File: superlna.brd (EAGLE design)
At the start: 41.2 x 21.8 mm, 14 parts, among them U1 BIASTEE, X1 SMA-142-0701-801/806, X2 SMA-142-0701-801/806

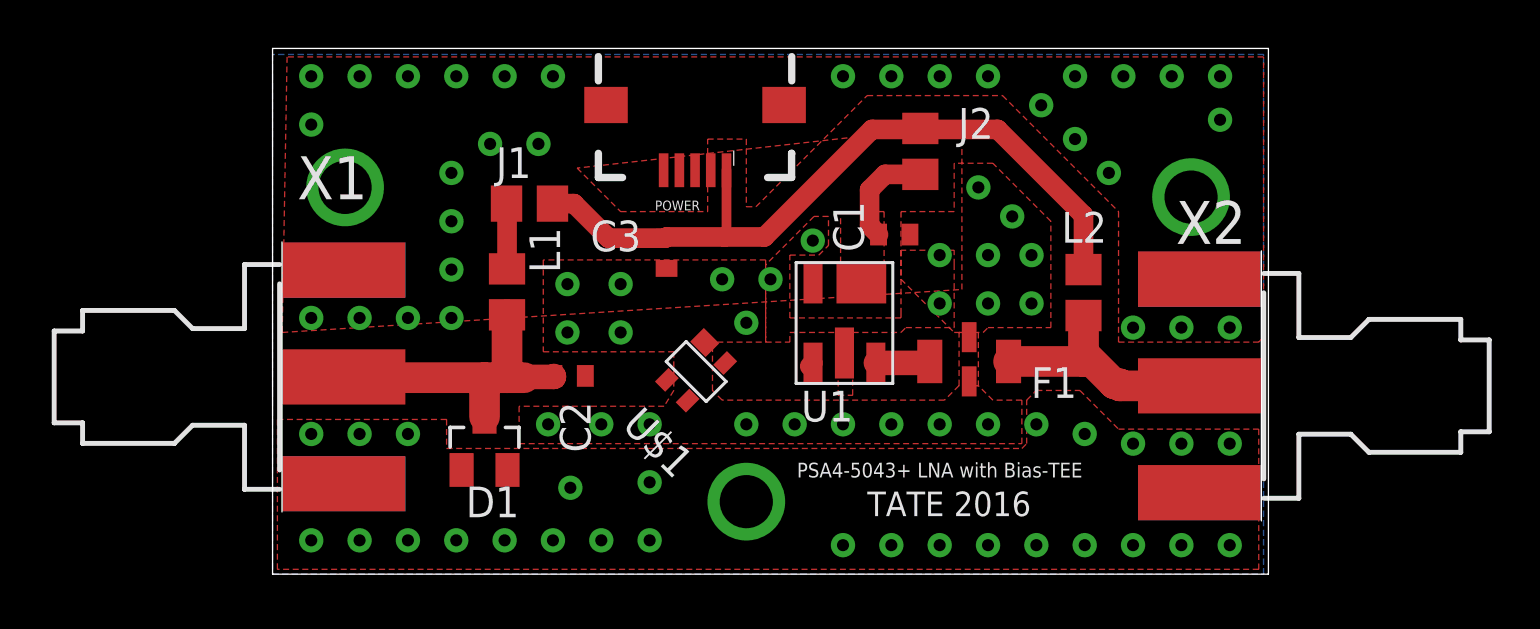
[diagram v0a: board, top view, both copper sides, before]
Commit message: V2
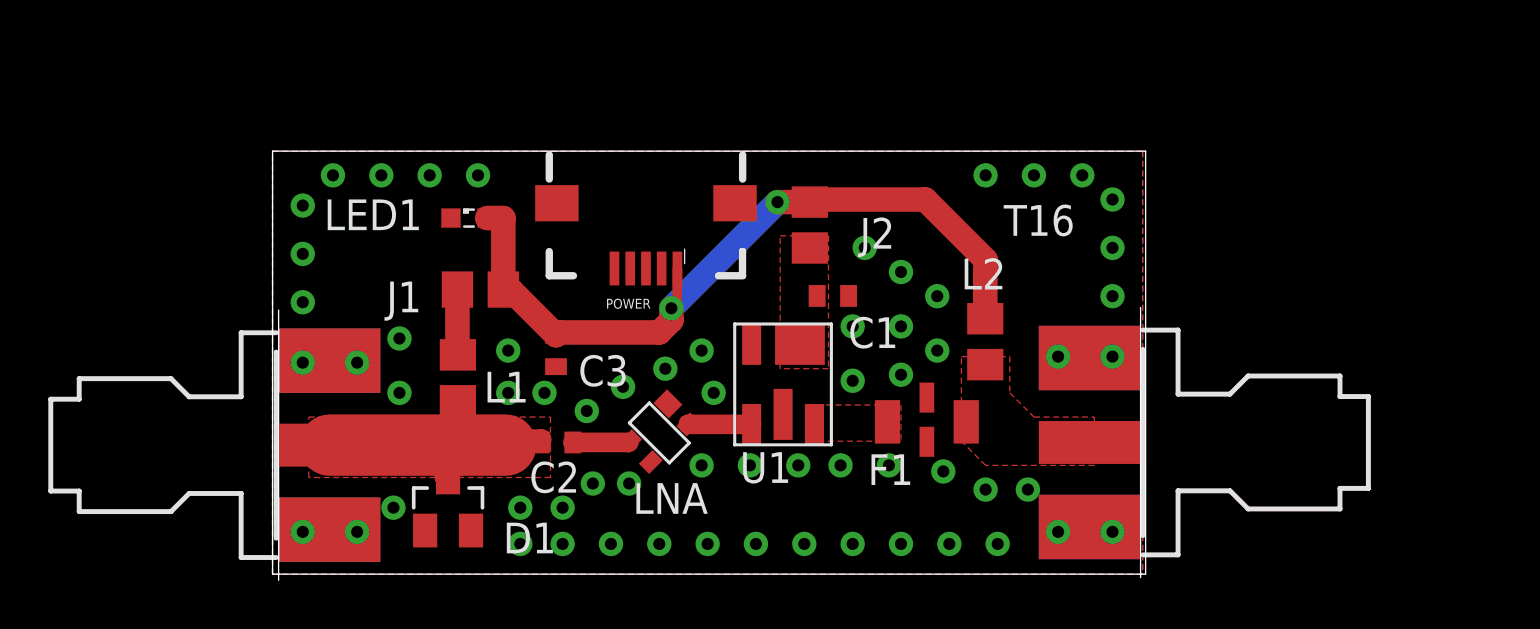
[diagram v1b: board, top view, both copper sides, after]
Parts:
- removed U$1: AMP, minicircuits:SOC-343
- removed X2: SMA-142-0701-801/806, con-coax:J502-ND-142-0701-801/806
- added LED1: (no value), eagle-ltspice:LED_SML0603
- added LNA: AMP, minicircuits:SOC-343
- added RFIN: SMA-142-0711-821/826, con-coax:J502-ND-142-0711-821/826
- X1: value SMA-142-0701-801/806 -> SMA-142-0711-821/826; device con-coax:J502-ND-142-0701-801/806 -> con-coax:J502-ND-142-0711-821/826
- moved X1 35.6 mm to (35.9, 5.45), turned to 180 degrees
- moved C3 6.12 mm to (11.7, 9.24)
- moved J2 5.49 mm to (22.2, 14.4)
- moved POWER 4.54 mm to (15.4, 15.3)
- moved L2 4.54 mm to (29.5, 9.62)
- moved J1 4.10 mm to (8.60, 11.8)
- moved L1 4.10 mm to (7.67, 8.12)
- moved C1 3.59 mm to (23.2, 11.5)
- moved U1 3.59 mm to (21.1, 7.85)
- moved F1 3.05 mm to (27.1, 6.39)
- moved D1 2.93 mm to (7.26, 2.90)
- moved C2 2.80 mm to (11.8, 5.45)
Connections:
- net N$6 renamed RFOUT1
- removed net N$4: C3.1, J1.1, J2.1, L2.1, POWER.VBUS1
- new net PWRIN: C3.1, J1.1, J2.1, L2.1, LED1.A, POWER.VBUS1
- net GND: now also LED1.C, LNA.GND, LNA.GND1, RFIN.G@1, RFIN.G@2, RFIN.G@3, RFIN.G@4; no longer U$1.GND, U$1.GND1, X2.G@1, X2.G@2, X2.G@3, X2.G@4
- net N$2: now also LNA.RFIN; no longer U$1.RFIN
- net N$5: now also LNA.RFOUT_DCIN; no longer U$1.RFOUT_DCIN
- net RFIN: now also RFIN.1; no longer X1.1
- net RFOUT: now also X1.1; no longer X2.1
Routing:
- net PWRIN: track 0.00 -> 32.2 mm, vias 0 -> 2
- net N$4: track 31.0 -> 0.00 mm
- net RFOUT: track 10.4 -> 0.00 mm
- net BIASPOWER: track 4.37 -> 0.00 mm
- net N$5: track 0.19 -> 2.62 mm
- net N$2: track 0.00 -> 2.39 mm
- net RFOUT1: track 2.25 -> 0.00 mm
- net RFIN: track 13.4 -> 12.5 mm
- added copper zone on layer 1, net RFIN
- added copper zone on layer 1, net RFOUT
- added copper zone on layer 1, net RFOUT1
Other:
- board size 41.2 x 21.8 mm -> 36.1 x 17.5 mm
- board text added: "T16"
- board text removed: "PSA4-5043+ LNA with Bias-TEE"
- board text removed: "TATE 2016"
